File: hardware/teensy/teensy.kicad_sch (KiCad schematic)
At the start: 83 parts, among them U1 Teensy3.5

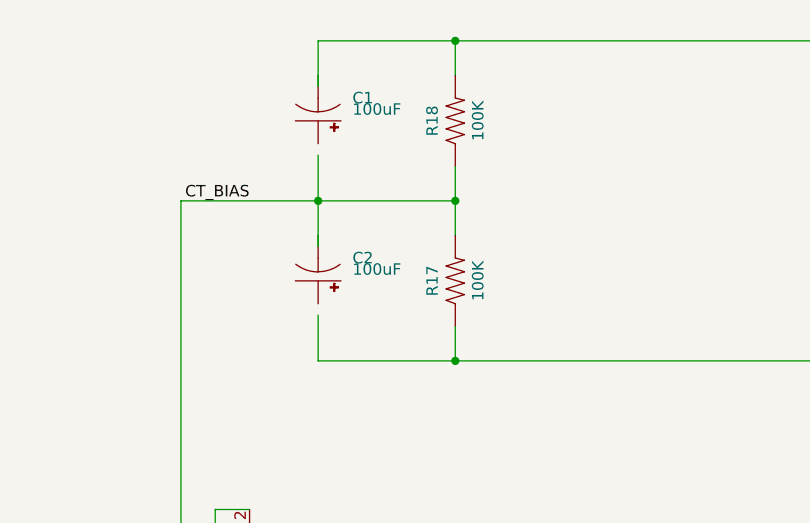
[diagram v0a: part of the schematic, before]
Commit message: fix the kicad, also tuning
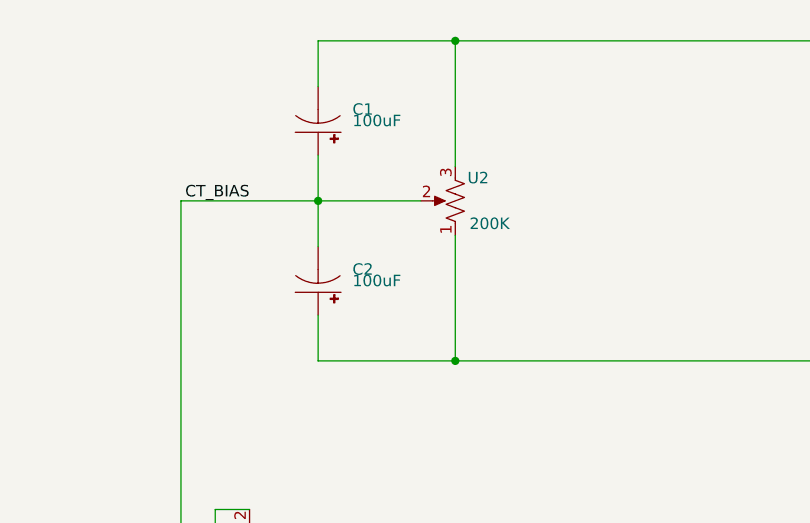
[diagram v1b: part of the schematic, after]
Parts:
- removed R17, R18: 100K, Resistors:AXIAL-0.3, symbol SparkFun-Resistors:RESISTORAXIAL-0.3
- added U2: 200K, Potentiometer_THT:Potentiometer_Bourns_3296W_Vertical, symbol Device:R_POT_US
- C1, C2: footprint Resistors:AXIAL-0.3 -> Capacitors:CPOL-RADIAL-5MM-10MM
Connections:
- net 3.3V: now also C2.+, U2.1
- net CT_BIAS: now also C1.+, C2.-, U2.2
- net GND: now also C1.-, U2.3
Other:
- moved on the sheet: C1, C2
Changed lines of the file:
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@@
   (junction (at 93.98 71.12) (diameter 0) (color 0 0 0 0))
   (junction (at 109.22 53.34) (diameter 0) (color 0 0 0 0))
-  (junction (at 109.22 71.12) (diameter 0) (color 0 0 0 0))
   (junction (at 109.22 88.9) (diameter 0) (color 0 0 0 0))
   (junction (at 109.22 109.22) (diameter 0) (color 0 0 0 0))
@@
     (stroke (width 0) (type solid) (color 0 0 0 0))
   )
-  (wire (pts (xy 93.98 71.12) (xy 109.22 71.12))
+  (wire (pts (xy 93.98 71.12) (xy 105.41 71.12))
     (stroke (width 0) (type solid) (color 0 0 0 0))
   )
@@
     (stroke (width 0) (type solid) (color 0 0 0 0))
   )
-  (wire (pts (xy 109.22 53.34) (xy 194.31 53.34))
-    (stroke (width 0) (type solid) (color 0 0 0 0))
-  )
-  (wire (pts (xy 109.22 57.15) (xy 109.22 53.34))
+  (wire (pts (xy 109.22 53.34) (xy 109.22 67.31))
     (stroke (width 0) (type solid) (color 0 0 0 0))
   )
-  (wire (pts (xy 109.22 71.12) (xy 109.22 67.31))
+  (wire (pts (xy 109.22 53.34) (xy 194.31 53.34))
     (stroke (width 0) (type solid) (color 0 0 0 0))
   )
-  (wire (pts (xy 109.22 74.93) (xy 109.22 71.12))
+  (wire (pts (xy 109.22 74.93) (xy 109.22 88.9))
     (stroke (width 0) (type solid) (color 0 0 0 0))
   )
@@
     (stroke (width 0) (type solid) (color 0 0 0 0))
   )
-  (wire (pts (xy 109.22 88.9) (xy 109.22 85.09))
-    (stroke (width 0) (type solid) (color 0 0 0 0))
-  )
   (wire (pts (xy 109.22 88.9) (xy 194.31 88.9))
     (stroke (width 0) (type solid) (color 0 0 0 0))
@@
     (effects (font (size 1.27 1.27)) (justify right bottom))
   )
-  (symbol (lib_id "SparkFun-Resistors:RESISTORAXIAL-0.3") (at 109.22 62.23 90) (unit 1)
-    (in_bom yes) (on_board yes)
-    (property "Reference" "R18" (id 0) (at 109.22 62.23 0)
-      (effects (font (size 1.27 1.27)) hide)
-    )
-    (property "Value" "100K" (id 1) (at 111.76 62.23 0))
-    (property "Footprint" "Resistors:AXIAL-0.3" (id 2) (at 109.22 62.23 0)
-      (effects (font (size 1.27 1.27)) hide)
-    )
-    (property "Datasheet" "" (id 3) (at 109.22 62.23 0)
-      (effects (font (size 1.27 1.27)) hide)
-    )
-    (property "Reference" "R18" (id 4) (at 106.68 62.23 0))
-    (property "Footprint" "Resistors:AXIAL-0.3" (id 6) (at 109.22 62.23 0)
-      (effects (font (size 1.27 1.27)) hide)
-    )
-    (property "Datasheet" "" (id 7) (at 109.22 62.23 0)
-      (effects (font (size 1.27 1.27)) hide)
-    )
-  )
-  (symbol (lib_id "SparkFun-Resistors:RESISTORAXIAL-0.3") (at 109.22 80.01 90) (unit 1)
-    (in_bom yes) (on_board yes)
-    (property "Reference" "R17" (id 0) (at 109.22 80.01 0)
-      (effects (font (size 1.27 1.27)) hide)
-    )
-    (property "Value" "100K" (id 1) (at 109.22 80.01 0)
-      (effects (font (size 1.27 1.27)) hide)
-    )
-    (property "Footprint" "Resistors:AXIAL-0.3" (id 2) (at 109.22 80.01 0)
-      (effects (font (size 1.27 1.27)) hide)
-    )
-    (property "Datasheet" "" (id 3) (at 109.22 80.01 0)
-      (effects (font (size 1.27 1.27)) hide)
-    )
-    (property "Reference" "R17" (id 4) (at 106.68 80.01 0))
-    (property "Value" "100K" (id 5) (at 111.76 80.01 0))
-    (property "Footprint" "Resistors:AXIAL-0.3" (id 6) (at 109.22 80.01 0)
-      (effects (font (size 1.27 1.27)) hide)
-    )
-    (property "Datasheet" "" (id 7) (at 109.22 80.01 0)
-      (effects (font (size 1.27 1.27)) hide)
-    )
-  )
   (symbol (lib_id "SparkFun-Resistors:RESISTORAXIAL-0.3") (at 148.59 109.22 0) (unit 1)
     (in_bom yes) (on_board yes)
@@
     )
   )
-  (symbol (lib_id "SparkFun-Capacitors:100UF-POLAR-10X10.5-63V-20%") (at 93.98 62.23 180) (unit 1)
+  (symbol (lib_id "SparkFun-Capacitors:100UF-POLAR-10X10.5-63V-20%") (at 93.98 63.5 180) (unit 1)
     (in_bom yes) (on_board yes)
-    (property "Reference" "C1" (id 0) (at 97.79 59.69 0)
+    (property "Reference" "C1" (id 0) (at 97.79 60.96 0)
       (effects (font (size 1.27 1.27)) (justify right))
     )
-    (property "Value" "100uF" (id 1) (at 97.79 60.96 0)
+    (property "Value" "100uF" (id 1) (at 97.79 62.23 0)
       (effects (font (size 1.27 1.27)) (justify right))
     )
-    (property "Footprint" "Resistors:AXIAL-0.3" (id 2) (at 93.98 62.23 0)
+    (property "Footprint" "Capacitors:CPOL-RADIAL-5MM-10MM" (id 2) (at 93.98 63.5 0)
       (effects (font (size 1.27 1.27)) hide)
     )
-    (property "Datasheet" "~" (id 3) (at 93.98 62.23 0)
+    (property "Datasheet" "~" (id 3) (at 93.98 63.5 0)
       (effects (font (size 1.27 1.27)) hide)
     )
   )
-  (symbol (lib_id "SparkFun-Capacitors:100UF-POLAR-10X10.5-63V-20%") (at 93.98 80.01 180) (unit 1)
+  (symbol (lib_id "SparkFun-Capacitors:100UF-POLAR-10X10.5-63V-20%") (at 93.98 81.28 180) (unit 1)
     (in_bom yes) (on_board yes)
-    (property "Reference" "C2" (id 0) (at 97.79 77.47 0)
+    (property "Reference" "C2" (id 0) (at 97.79 78.74 0)
       (effects (font (size 1.27 1.27)) (justify right))
     )
-    (property "Value" "100uF" (id 1) (at 97.79 78.74 0)
+    (property "Value" "100uF" (id 1) (at 97.79 80.01 0)
       (effects (font (size 1.27 1.27)) (justify right))
     )
-    (property "Footprint" "Resistors:AXIAL-0.3" (id 2) (at 93.98 80.01 0)
+    (property "Footprint" "Capacitors:CPOL-RADIAL-5MM-10MM" (id 2) (at 93.98 81.28 0)
       (effects (font (size 1.27 1.27)) hide)
     )
-    (property "Datasheet" "~" (id 3) (at 93.98 80.01 0)
+    (property "Datasheet" "~" (id 3) (at 93.98 81.28 0)
       (effects (font (size 1.27 1.27)) hide)
     )
@@
     )
   )
+  (symbol (lib_id "Device:R_POT_US") (at 109.22 71.12 180) (unit 1)
+    (in_bom yes) (on_board yes)
+    (property "Reference" "U2" (id 0) (at 111.76 68.58 0))
+    (property "Value" "200K" (id 1) (at 113.03 73.66 0))
+    (property "Footprint" "Potentiometer_THT:Potentiometer_Bourns_3296W_Vertical" (id 2) (at 109.22 71.12 0)
+      (effects (font (size 1.27 1.27)) hide)
+    )
+    (property "Datasheet" "" (id 3) (at 109.22 71.12 0)
+      (effects (font (size 1.27 1.27)) hide)
+    )
+  )
   (symbol (lib_id "SparkFun-Connectors:CONN_08NO_SILK_FEMALE_PTH") (at 58.42 127 0) (unit 1)
     (in_bom yes) (on_board yes)
@@
       (reference "J6") (unit 1)
     )
-    (path "/9898e971-41cc-490c-a439-0d9d80299fa0"
-      (reference "R17") (unit 1)
-    )
-    (path "/eab86b04-2b47-4fd3-9787-6b1023ff96d9"
-      (reference "R18") (unit 1)
-    )
     (path "/906a0f35-4b46-4202-9289-e26007a61c26"
       (reference "R23") (unit 1)
@@
       (reference "U1") (unit 1)
     )
+    (path "/b41b3177-9c6e-478c-8b8e-c9ef4791192b"
+      (reference "U2") (unit 1)
+    )
   )
